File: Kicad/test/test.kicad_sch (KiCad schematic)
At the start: 74 parts, among them J1 SPKOUT, J2 Tag Con, P1 USB_C_Plug_USB2.0, SW2 SW_Push, SW3 SW_Push, SW4 SW_Push, SW5 SW_Push, U1 MAX98357A, U2 ESP32-S3-WROOM-1, U3 OV5640, U4 24Mhz, U5 AXP2101

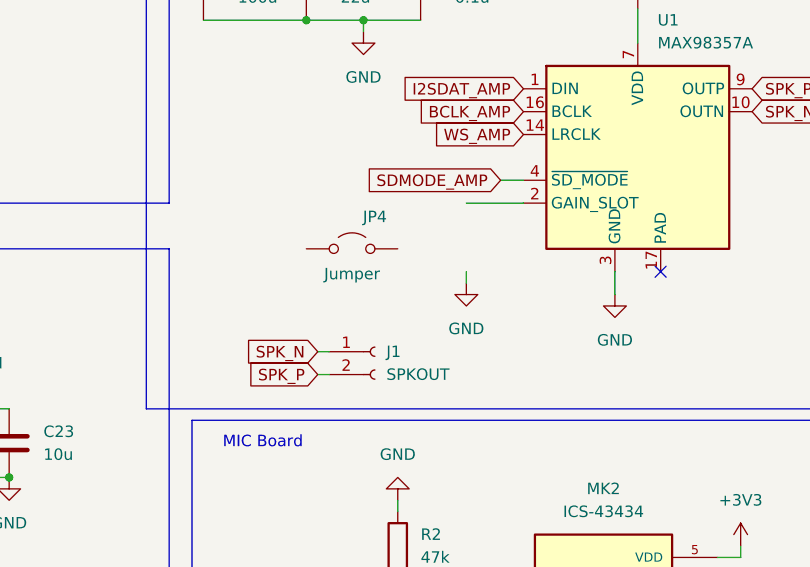
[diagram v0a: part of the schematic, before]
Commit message: Connected a missing piece
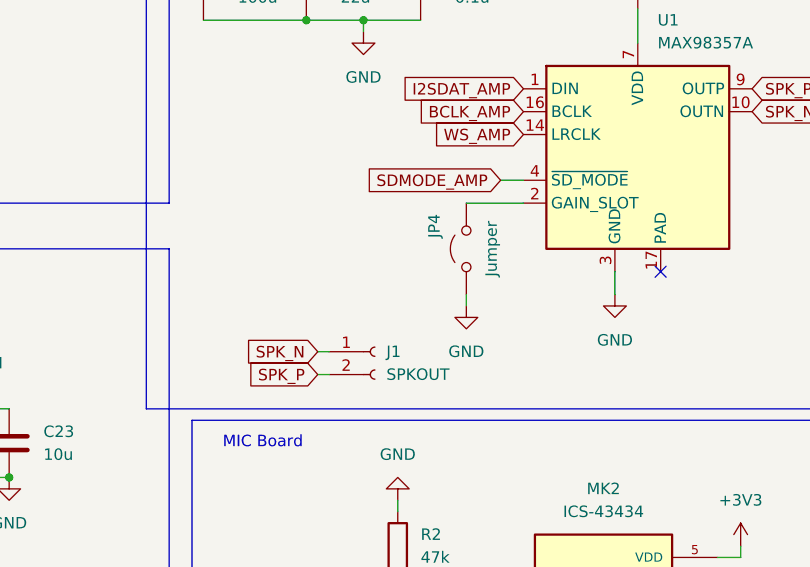
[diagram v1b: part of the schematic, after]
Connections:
- net GND: now also JP4.1 (A)
- net at U1.2 (GAIN_SLOT): now also JP4.2 (B)
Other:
- moved on the sheet: JP4
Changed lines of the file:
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@@
 	(wire
 		(pts
+			(xy 220.98 219.71) (xy 220.98 220.98)
+		)
+		(stroke
+			(width 0)
+			(type default)
+		)
+	)
+	(wire
+		(pts
 			(xy 71.12 186.69) (xy 71.12 185.42)
 		)
@@
 	(wire
 		(pts
-			(xy 220.98 217.17) (xy 220.98 218.44)
-		)
-		(stroke
-			(width 0)
-			(type default)
-		)
-	)
-	(wire
-		(pts
 			(xy 111.76 266.7) (xy 111.76 275.59)
 		)
@@
 	(symbol
 		(lib_id "power:GND")
-		(at 220.98 218.44 0)
+		(at 220.98 220.98 0)
 		(unit 1)
 		(exclude_from_sim no)
@@
 		(fields_autoplaced yes)
 		(property "Reference" "#PWR017"
-			(at 220.98 224.79 0)
+			(at 220.98 227.33 0)
 			(effects
 				(font
@@
 		)
 		(property "Value" "GND"
-			(at 220.98 223.52 0)
+			(at 220.98 226.06 0)
 			(effects
 				(font
@@
 		)
 		(property "Footprint" ""
-			(at 220.98 218.44 0)
+			(at 220.98 220.98 0)
 			(effects
 				(font
@@
 		)
 		(property "Datasheet" ""
-			(at 220.98 218.44 0)
+			(at 220.98 220.98 0)
 			(effects
 				(font
@@
 		)
 		(property "Description" "Power symbol creates a global label with name \"GND\" , ground"
-			(at 220.98 218.44 0)
+			(at 220.98 220.98 0)
 			(effects
 				(font
@@
 	(symbol
 		(lib_id "Jumper:Jumper_2_Open")
-		(at 208.28 214.63 0)
+		(at 220.98 214.63 90)
 		(unit 1)
 		(exclude_from_sim yes)
@@
 		(dnp no)
 		(property "Reference" "JP4"
-			(at 210.82 211.074 0)
+			(at 217.424 212.09 0)
 			(effects
 				(font
@@
 		)
 		(property "Value" "Jumper"
-			(at 208.28 217.424 0)
+			(at 223.774 214.63 0)
 			(effects
 				(font
@@
 		)
 		(property "Footprint" "Jumper:SolderJumper-2_P1.3mm_Open_TrianglePad1.0x1.5mm"
-			(at 208.28 214.63 0)
+			(at 220.98 214.63 0)
 			(effects
 				(font
@@
 		)
 		(property "Datasheet" "~"
-			(at 208.28 214.63 0)
+			(at 220.98 214.63 0)
 			(effects
 				(font
@@
 		)
 		(property "Description" "Jumper, 2-pole, open"
-			(at 208.28 214.63 0)
+			(at 220.98 214.63 0)
 			(effects
 				(font

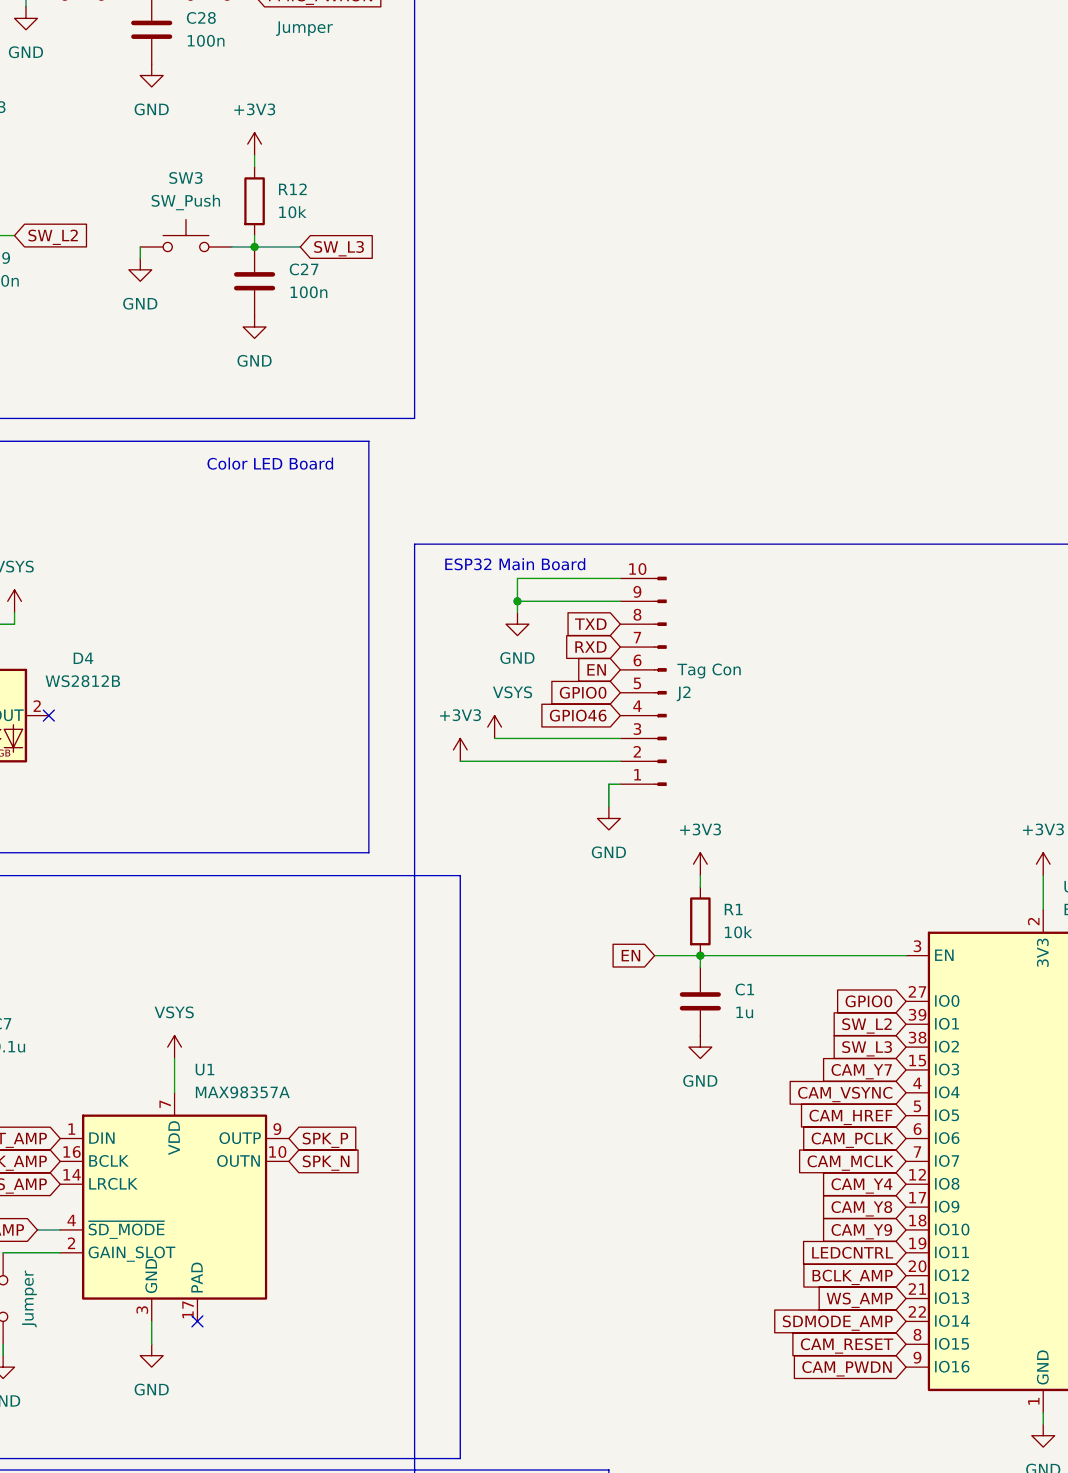
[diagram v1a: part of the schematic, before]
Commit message: 50% Routing Done
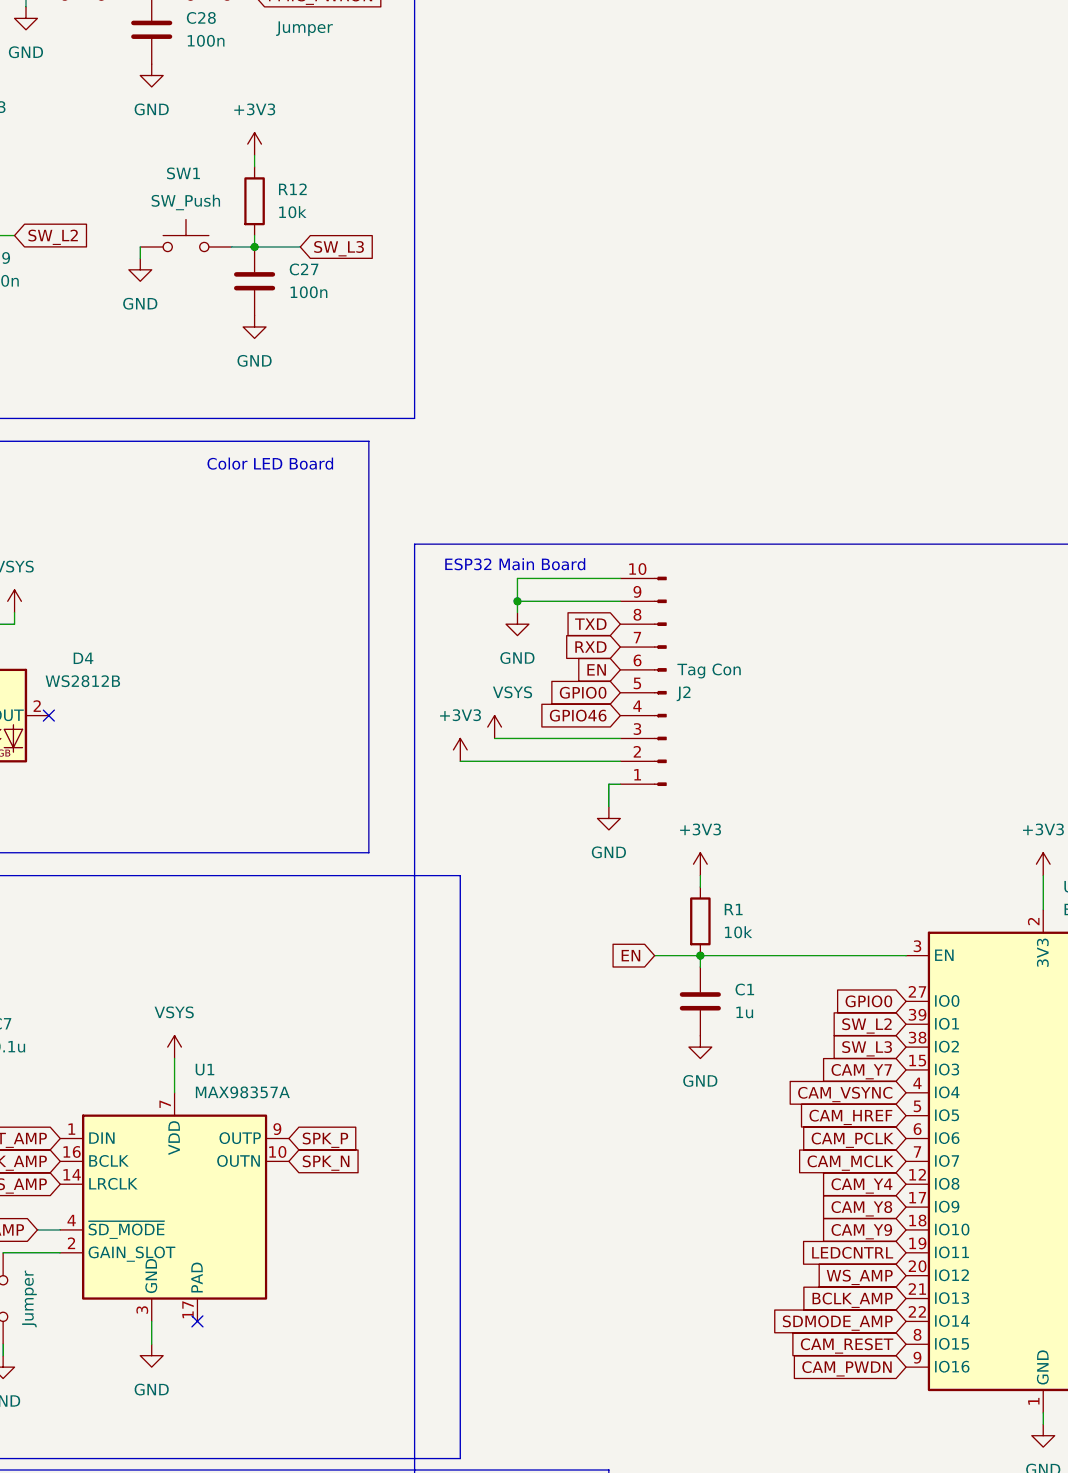
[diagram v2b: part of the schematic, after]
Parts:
- removed SW3: SW_Push, switchLibrary:K2-1114SA-A4SW-06, symbol Switch:SW_Push
- added SW1: SW_Push, Library:SW2_1825027-C_TEC, symbol Switch:SW_Push
- SW2: footprint switchLibrary:K2-1114SA-A4SW-06 -> Library:SW2_1825027-C_TEC; LCSC Part C136662 -> C266196; Mfr Part K2-1114SA-A4SW-06 -> 1825027-8
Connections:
- net BCLK_AMP: now also U2.21 (IO13); no longer U2.20 (IO12)
- net GND: now also SW1.1
- net SW_L3: now also SW1.2
- net WS_AMP: now also U2.20 (IO12); no longer U2.21 (IO13)
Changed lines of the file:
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@@
 	(global_label "WS_AMP"
 		(shape input)
-		(at 321.31 214.63 180)
+		(at 321.31 212.09 180)
 		(fields_autoplaced yes)
 		(effects
@@
 		)
 		(property "Intersheetrefs" "${INTERSHEET_REFS}"
-			(at 310.8863 214.63 0)
+			(at 310.8863 212.09 0)
 			(effects
 				(font
@@
 	(global_label "BCLK_AMP"
 		(shape input)
-		(at 321.31 212.09 180)
+		(at 321.31 214.63 180)
 		(fields_autoplaced yes)
 		(effects
@@
 		)
 		(property "Intersheetrefs" "${INTERSHEET_REFS}"
-			(at 308.7091 212.09 0)
+			(at 308.7091 214.63 0)
 			(effects
 				(font
@@
 	)
 	(symbol
+		(lib_id "Switch:SW_Push")
+		(at 241.3 97.79 0)
+		(unit 1)
+		(exclude_from_sim no)
+		(in_bom yes)
+		(on_board yes)
+		(dnp no)
+		(property "Reference" "SW1"
+			(at 241.046 89.662 0)
+			(effects
+				(font
+					(size 1.27 1.27)
+				)
+			)
+		)
+		(property "Value" "SW_Push"
+			(at 241.3 92.71 0)
+			(effects
+				(font
+					(size 1.27 1.27)
+				)
+			)
+		)
+		(property "Footprint" "Library:SW2_1825027-C_TEC"
+			(at 241.3 92.71 0)
+			(effects
+				(font
+					(size 1.27 1.27)
+				)
+				(hide yes)
+			)
+		)
+		(property "Datasheet" "https://www.lcsc.com/datasheet/lcsc_datasheet_2411220707_TE-Connectivity-1825027-8_C266196.pdf"
+			(at 241.3 92.71 0)
+			(effects
+				(font
+					(size 1.27 1.27)
+				)
+				(hide yes)
+			)
+		)
+		(property "Description" "3.25mm Round Button 50mA Bend-in SPST 160gf 24V Plugin Tactile Switches ROHS"
+			(at 241.3 97.79 0)
+			(effects
+				(font
+					(size 1.27 1.27)
+				)
+				(hide yes)
+			)
+		)
+		(property "LCSC Part" "C266196"
+			(at 241.3 97.79 0)
+			(effects
+				(font
+					(size 1.27 1.27)
+				)
+				(hide yes)
+			)
+		)
+		(property "Mfr Part" "1825027-8"
+			(at 241.3 97.79 0)
+			(effects
+				(font
+					(size 1.27 1.27)
+				)
+				(hide yes)
+			)
+		)
+		(pin "1"
+		)
+		(pin "2"
+		)
+		(instances
+			(project "test"
+				(path "/2b9d0de6-8b12-4765-99af-867ac9f145de"
+					(reference "SW1")
+					(unit 1)
+				)
+			)
+		)
+	)
+	(symbol
 		(lib_id "power:GND")
 		(at 288.29 160.02 0)
@@
 	)
 	(symbol
-		(lib_id "Switch:SW_Push")
-		(at 241.3 97.79 0)
-		(unit 1)
-		(exclude_from_sim no)
-		(in_bom yes)
-		(on_board yes)
-		(dnp no)
-		(fields_autoplaced yes)
-		(property "Reference" "SW3"
-			(at 241.3 90.17 0)
-			(effects
-				(font
-					(size 1.27 1.27)
-				)
-			)
-		)
-		(property "Value" "SW_Push"
-			(at 241.3 92.71 0)
-			(effects
-				(font
-					(size 1.27 1.27)
-				)
-			)
-		)
-		(property "Footprint" "switchLibrary:K2-1114SA-A4SW-06"
-			(at 241.3 92.71 0)
-			(effects
-				(font
-					(size 1.27 1.27)
-				)
-				(hide yes)
-			)
-		)
-		(property "Datasheet" "https://www.lcsc.com/datasheet/lcsc_datasheet_1810061013_Korean-Hroparts-Elec-K2-1114SA-A4SW-06_C136662.pdf"
-			(at 241.3 92.71 0)
-			(effects
-				(font
-					(size 1.27 1.27)
-				)
-				(hide yes)
-			)
-		)
-		(property "Description" "3.5mm 1.65mm Rectangle button 50mA Horizontal attachment 4.8mm SPST 100000 Times 250gf 12V SMD Tactile Switches ROHS"
-			(at 241.3 97.79 0)
-			(effects
-				(font
-					(size 1.27 1.27)
-				)
-				(hide yes)
-			)
-		)
-		(property "LCSC Part" "C136662"
-			(at 241.3 97.79 0)
-			(effects
-				(font
-					(size 1.27 1.27)
-				)
-				(hide yes)
-			)
-		)
-		(property "Mfr Part" "K2-1114SA-A4SW-06"
-			(at 241.3 97.79 0)
-			(effects
-				(font
-					(size 1.27 1.27)
-				)
-				(hide yes)
-			)
-		)
-		(pin "1"
-		)
-		(pin "2"
-		)
-		(instances
-			(project "test"
-				(path "/2b9d0de6-8b12-4765-99af-867ac9f145de"
-					(reference "SW3")
-					(unit 1)
-				)
-			)
-		)
-	)
-	(symbol
 		(lib_id "power:+1V5")
 		(at 66.04 186.69 0)
@@
 			)
 		)
-		(property "Footprint" "switchLibrary:K2-1114SA-A4SW-06"
+		(property "Footprint" "Library:SW2_1825027-C_TEC"
 			(at 201.93 91.44 0)
 			(effects
@@
 			)
 		)
-		(property "Datasheet" "https://www.lcsc.com/datasheet/lcsc_datasheet_1810061013_Korean-Hroparts-Elec-K2-1114SA-A4SW-06_C136662.pdf"
+		(property "Datasheet" "https://www.lcsc.com/datasheet/lcsc_datasheet_2411220707_TE-Connectivity-1825027-8_C266196.pdf"
 			(at 201.93 91.44 0)
 			(effects
@@
 			)
 		)
-		(property "Description" "3.5mm 1.65mm Rectangle button 50mA Horizontal attachment 4.8mm SPST 100000 Times 250gf 12V SMD Tactile Switches ROHS"
+		(property "Description" "3.25mm Round Button 50mA Bend-in SPST 160gf 24V Plugin Tactile Switches ROHS"
 			(at 201.93 96.52 0)
 			(effects
@@
 			)
 		)
-		(property "LCSC Part" "C136662"
+		(property "LCSC Part" "C266196"
 			(at 201.93 96.52 0)
 			(effects
@@
 			)
 		)
-		(property "Mfr Part" "K2-1114SA-A4SW-06"
+		(property "Mfr Part" "1825027-8"
 			(at 201.93 96.52 0)
 			(effects
